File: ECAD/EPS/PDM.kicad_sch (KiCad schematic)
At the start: 12 parts, among them Q30 2N7002, Q31 IRF7458, U24 INA180A3

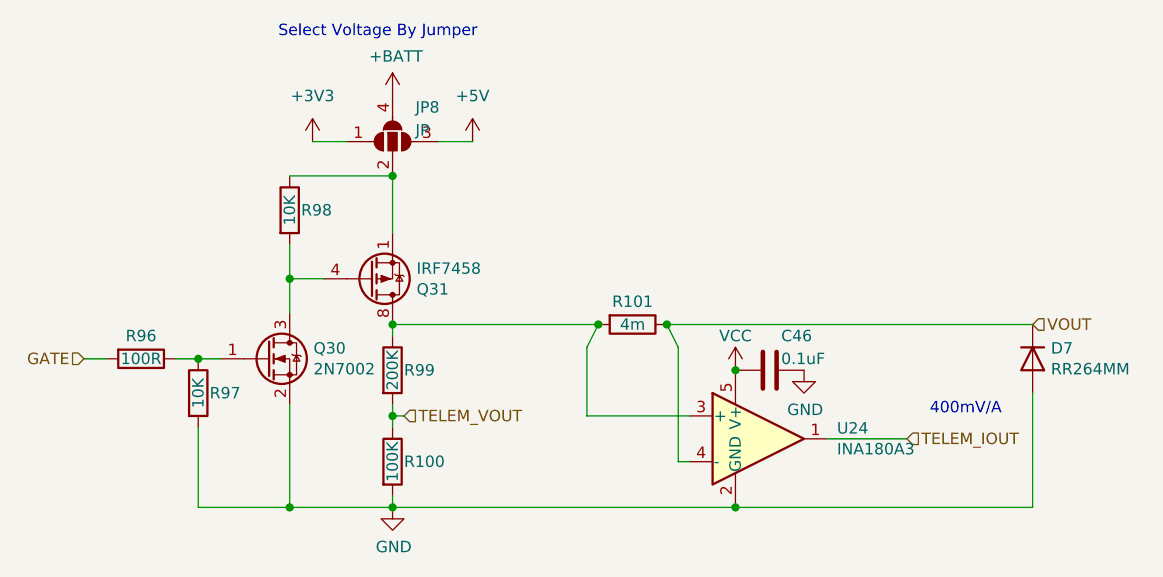
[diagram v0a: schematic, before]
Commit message: Micro + PCM blocks
Micro + PCM blocks
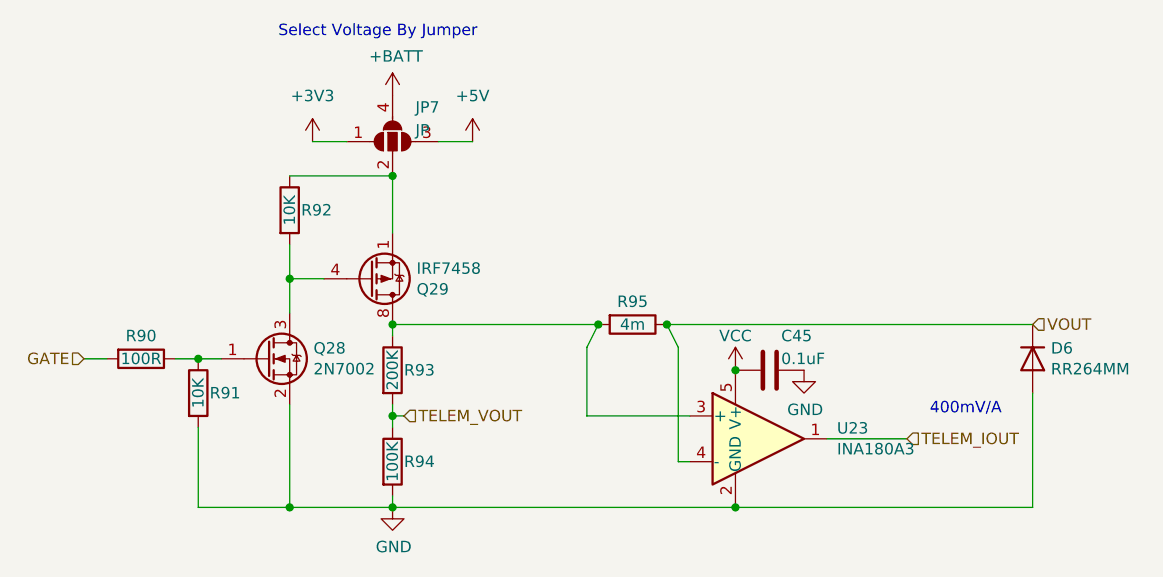
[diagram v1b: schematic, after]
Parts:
- renumbered C46 to C45, D7 to D6, JP8 to JP7, Q30 to Q28, Q31 to Q29, R96 to R90, R97 to R91, R98 to R92, R99 to R93, R100 to R94, R101 to R95, U24 to U23
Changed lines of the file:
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@@
     (effects (font (size 1.27 1.27)) (justify left))
   )
-  (symbol (lib_id "Device:D") (at 189.23 63.5 270) (unit 1)
-    (in_bom yes) (on_board yes)
-    (property "Reference" "D7" (id 0) (at 191.262 62.3316 90)
+  (symbol (lib_id "Device:D") (at 189.23 63.5 270)
+    (in_bom yes) (on_board yes)
+    (property "Reference" "D6" (id 0) (at 191.262 62.3316 90)
       (effects (font (size 1.27 1.27)) (justify left))
     )
@@
     (pin "2")
   )
-  (symbol (lib_id "Device:R") (at 118.11 64.77 0) (unit 1)
-    (in_bom yes) (on_board yes)
-    (property "Reference" "R99" (id 0) (at 119.38 64.77 0)
+  (symbol (lib_id "Device:R") (at 118.11 64.77 0)
+    (in_bom yes) (on_board yes)
+    (property "Reference" "R93" (id 0) (at 119.38 64.77 0)
       (effects (font (size 1.27 1.27)) (justify left))
     )
@@
     (pin "2")
   )
-  (symbol (lib_id "power:+BATT") (at 118.11 34.29 0) (unit 1)
-    (in_bom yes) (on_board yes)
-    (property "Reference" "#PWR0105" (id 0) (at 118.11 38.1 0)
+  (symbol (lib_id "power:+BATT") (at 118.11 34.29 0)
+    (in_bom yes) (on_board yes)
+    (property "Reference" "#PWR099" (id 0) (at 118.11 38.1 0)
       (effects (font (size 1.27 1.27)) hide)
     )
@@
     (pin "1")
   )
-  (symbol (lib_id "Transistor_FET:IRF7404") (at 115.57 54.61 0) (mirror x) (unit 1)
-    (in_bom yes) (on_board yes)
-    (property "Reference" "Q31" (id 0) (at 120.777 55.7784 0)
+  (symbol (lib_id "Transistor_FET:IRF7404") (at 115.57 54.61 0) (mirror x)
+    (in_bom yes) (on_board yes)
+    (property "Reference" "Q29" (id 0) (at 120.777 55.7784 0)
       (effects (font (size 1.27 1.27)) (justify left))
     )
@@
     (pin "8")
   )
-  (symbol (lib_id "Transistor_FET:2N7002") (at 104.14 63.5 0) (unit 1)
-    (in_bom yes) (on_board yes)
-    (property "Reference" "Q30" (id 0) (at 109.3216 62.3316 0)
+  (symbol (lib_id "Transistor_FET:2N7002") (at 104.14 63.5 0)
+    (in_bom yes) (on_board yes)
+    (property "Reference" "Q28" (id 0) (at 109.3216 62.3316 0)
       (effects (font (size 1.27 1.27)) (justify left))
     )
@@
     (pin "3")
   )
-  (symbol (lib_id "Device:R") (at 106.68 46.99 0) (unit 1)
-    (in_bom yes) (on_board yes)
-    (property "Reference" "R98" (id 0) (at 107.95 46.99 0)
+  (symbol (lib_id "Device:R") (at 106.68 46.99 0)
+    (in_bom yes) (on_board yes)
+    (property "Reference" "R92" (id 0) (at 107.95 46.99 0)
       (effects (font (size 1.27 1.27)) (justify left))
     )
@@
     (pin "2")
   )
-  (symbol (lib_id "Device:R") (at 90.17 63.5 270) (unit 1)
-    (in_bom yes) (on_board yes)
-    (property "Reference" "R96" (id 0) (at 90.17 60.96 90))
+  (symbol (lib_id "Device:R") (at 90.17 63.5 270)
+    (in_bom yes) (on_board yes)
+    (property "Reference" "R90" (id 0) (at 90.17 60.96 90))
     (property "Value" "100R" (id 1) (at 90.17 63.5 90))
     (property "Footprint" "" (id 2) (at 90.17 61.722 90)
@@
     (pin "2")
   )
-  (symbol (lib_id "Device:R") (at 96.52 67.31 0) (unit 1)
-    (in_bom yes) (on_board yes)
-    (property "Reference" "R97" (id 0) (at 97.79 67.31 0)
+  (symbol (lib_id "Device:R") (at 96.52 67.31 0)
+    (in_bom yes) (on_board yes)
+    (property "Reference" "R91" (id 0) (at 97.79 67.31 0)
       (effects (font (size 1.27 1.27)) (justify left))
     )
@@
     (pin "2")
   )
-  (symbol (lib_id "power:GND") (at 118.11 80.01 0) (unit 1)
-    (in_bom yes) (on_board yes)
-    (property "Reference" "#PWR0106" (id 0) (at 118.11 86.36 0)
+  (symbol (lib_id "power:GND") (at 118.11 80.01 0)
+    (in_bom yes) (on_board yes)
+    (property "Reference" "#PWR0100" (id 0) (at 118.11 86.36 0)
       (effects (font (size 1.27 1.27)) hide)
     )
@@
     (pin "1")
   )
-  (symbol (lib_id "Device:R") (at 144.78 59.69 270) (unit 1)
-    (in_bom yes) (on_board yes)
-    (property "Reference" "R101" (id 0) (at 144.78 57.15 90))
+  (symbol (lib_id "Device:R") (at 144.78 59.69 270)
+    (in_bom yes) (on_board yes)
+    (property "Reference" "R95" (id 0) (at 144.78 57.15 90))
     (property "Value" "4m" (id 1) (at 144.78 59.69 90))
     (property "Footprint" "Resistor_SMD:R_1206_3216Metric" (id 2) (at 144.78 57.912 90)
@@
     (pin "2")
   )
-  (symbol (lib_id "Device:R") (at 118.11 74.93 0) (unit 1)
-    (in_bom yes) (on_board yes)
-    (property "Reference" "R100" (id 0) (at 119.38 74.93 0)
+  (symbol (lib_id "Device:R") (at 118.11 74.93 0)
+    (in_bom yes) (on_board yes)
+    (property "Reference" "R94" (id 0) (at 119.38 74.93 0)
       (effects (font (size 1.27 1.27)) (justify left))
     )
@@
     (pin "2")
   )
-  (symbol (lib_id "Amplifier_Current:INA138") (at 158.75 72.39 0) (unit 1)
-    (in_bom yes) (on_board yes)
-    (property "Reference" "U24" (id 0) (at 167.4876 71.2216 0)
+  (symbol (lib_id "Amplifier_Current:INA138") (at 158.75 72.39 0)
+    (in_bom yes) (on_board yes)
+    (property "Reference" "U23" (id 0) (at 167.4876 71.2216 0)
       (effects (font (size 1.27 1.27)) (justify left))
     )
@@
     (pin "5")
   )
-  (symbol (lib_id "power:VCC") (at 156.21 64.77 0) (unit 1)
-    (in_bom yes) (on_board yes)
-    (property "Reference" "#PWR0108" (id 0) (at 156.21 68.58 0)
+  (symbol (lib_id "power:VCC") (at 156.21 64.77 0)
+    (in_bom yes) (on_board yes)
+    (property "Reference" "#PWR0102" (id 0) (at 156.21 68.58 0)
       (effects (font (size 1.27 1.27)) hide)
     )
@@
     (pin "1")
   )
-  (symbol (lib_id "Device:C") (at 160.02 64.77 90) (unit 1)
-    (in_bom yes) (on_board yes)
-    (property "Reference" "C46" (id 0) (at 161.29 60.96 90)
+  (symbol (lib_id "Device:C") (at 160.02 64.77 90)
+    (in_bom yes) (on_board yes)
+    (property "Reference" "C45" (id 0) (at 161.29 60.96 90)
       (effects (font (size 1.27 1.27)) (justify right))
     )
@@
     (pin "2")
   )
-  (symbol (lib_id "power:GND") (at 163.83 64.77 0) (unit 1)
-    (in_bom yes) (on_board yes)
-    (property "Reference" "#PWR0109" (id 0) (at 163.83 71.12 0)
+  (symbol (lib_id "power:GND") (at 163.83 64.77 0)
+    (in_bom yes) (on_board yes)
+    (property "Reference" "#PWR0103" (id 0) (at 163.83 71.12 0)
       (effects (font (size 1.27 1.27)) hide)
     )
@@
     (pin "1")
   )
-  (symbol (lib_id "symbols:SolderJumper_4_Open") (at 118.11 39.37 0) (unit 1)
-    (in_bom yes) (on_board yes)
-    (property "Reference" "JP8" (id 0) (at 120.65 35.56 0)
+  (symbol (lib_id "symbols:SolderJumper_4_Open") (at 118.11 39.37 0)
+    (in_bom yes) (on_board yes)
+    (property "Reference" "JP7" (id 0) (at 120.65 35.56 0)
       (effects (font (size 1.27 1.27)) (justify left))
     )
@@
     (pin "4")
   )
-  (symbol (lib_id "power:+5V") (at 127 39.37 0) (unit 1)
+  (symbol (lib_id "power:+5V") (at 127 39.37 0)
     (in_bom yes) (on_board yes) (fields_autoplaced)
-    (property "Reference" "#PWR0107" (id 0) (at 127 43.18 0)
+    (property "Reference" "#PWR0101" (id 0) (at 127 43.18 0)
       (effects (font (size 1.27 1.27)) hide)
     )
@@
     (pin "1")
   )
-  (symbol (lib_id "power:+3V3") (at 109.22 39.37 0) (unit 1)
+  (symbol (lib_id "power:+3V3") (at 109.22 39.37 0)
     (in_bom yes) (on_board yes) (fields_autoplaced)
-    (property "Reference" "#PWR0104" (id 0) (at 109.22 43.18 0)
-      (effects (font (size 1.27 1.27)) hide)
-    )
+    (property "Reference" "#PWR098" (id 0) (at 109.22 43.18 0)
+      (effects (font (size 1.27 1.27)) hide)
+    )

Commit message: Revert "Micro + PCM blocks"
This reverts commit bd53ca95fb26b4e6798500a23db46c8297649bcb.
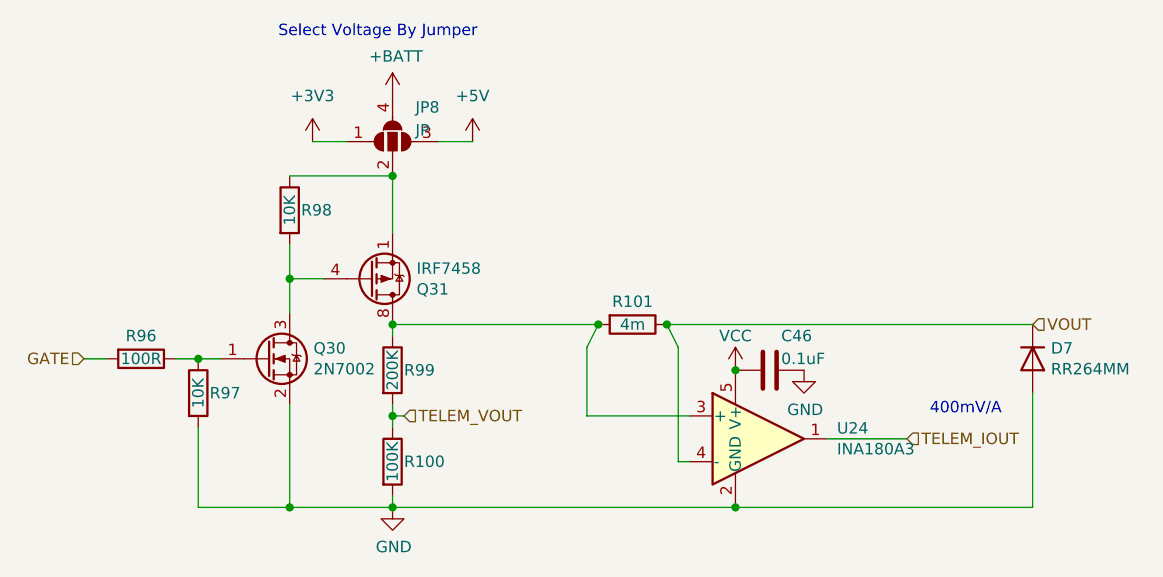
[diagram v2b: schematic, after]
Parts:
- renumbered C45 to C46, D6 to D7, JP7 to JP8, Q28 to Q30, Q29 to Q31, R94 to R100, R95 to R101, R90 to R96, R91 to R97, R92 to R98, R93 to R99, U23 to U24
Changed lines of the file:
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@@
     (effects (font (size 1.27 1.27)) (justify left))
   )
-  (symbol (lib_id "Device:D") (at 189.23 63.5 270)
-    (in_bom yes) (on_board yes)
-    (property "Reference" "D6" (id 0) (at 191.262 62.3316 90)
+  (symbol (lib_id "Device:D") (at 189.23 63.5 270) (unit 1)
+    (in_bom yes) (on_board yes)
+    (property "Reference" "D7" (id 0) (at 191.262 62.3316 90)
       (effects (font (size 1.27 1.27)) (justify left))
     )
@@
     (pin "2")
   )
-  (symbol (lib_id "Device:R") (at 118.11 64.77 0)
-    (in_bom yes) (on_board yes)
-    (property "Reference" "R93" (id 0) (at 119.38 64.77 0)
+  (symbol (lib_id "Device:R") (at 118.11 64.77 0) (unit 1)
+    (in_bom yes) (on_board yes)
+    (property "Reference" "R99" (id 0) (at 119.38 64.77 0)
       (effects (font (size 1.27 1.27)) (justify left))
     )
@@
     (pin "2")
   )
-  (symbol (lib_id "power:+BATT") (at 118.11 34.29 0)
-    (in_bom yes) (on_board yes)
-    (property "Reference" "#PWR099" (id 0) (at 118.11 38.1 0)
+  (symbol (lib_id "power:+BATT") (at 118.11 34.29 0) (unit 1)
+    (in_bom yes) (on_board yes)
+    (property "Reference" "#PWR0105" (id 0) (at 118.11 38.1 0)
       (effects (font (size 1.27 1.27)) hide)
     )
@@
     (pin "1")
   )
-  (symbol (lib_id "Transistor_FET:IRF7404") (at 115.57 54.61 0) (mirror x)
-    (in_bom yes) (on_board yes)
-    (property "Reference" "Q29" (id 0) (at 120.777 55.7784 0)
+  (symbol (lib_id "Transistor_FET:IRF7404") (at 115.57 54.61 0) (mirror x) (unit 1)
+    (in_bom yes) (on_board yes)
+    (property "Reference" "Q31" (id 0) (at 120.777 55.7784 0)
       (effects (font (size 1.27 1.27)) (justify left))
     )
@@
     (pin "8")
   )
-  (symbol (lib_id "Transistor_FET:2N7002") (at 104.14 63.5 0)
-    (in_bom yes) (on_board yes)
-    (property "Reference" "Q28" (id 0) (at 109.3216 62.3316 0)
+  (symbol (lib_id "Transistor_FET:2N7002") (at 104.14 63.5 0) (unit 1)
+    (in_bom yes) (on_board yes)
+    (property "Reference" "Q30" (id 0) (at 109.3216 62.3316 0)
       (effects (font (size 1.27 1.27)) (justify left))
     )
@@
     (pin "3")
   )
-  (symbol (lib_id "Device:R") (at 106.68 46.99 0)
-    (in_bom yes) (on_board yes)
-    (property "Reference" "R92" (id 0) (at 107.95 46.99 0)
+  (symbol (lib_id "Device:R") (at 106.68 46.99 0) (unit 1)
+    (in_bom yes) (on_board yes)
+    (property "Reference" "R98" (id 0) (at 107.95 46.99 0)
       (effects (font (size 1.27 1.27)) (justify left))
     )
@@
     (pin "2")
   )
-  (symbol (lib_id "Device:R") (at 90.17 63.5 270)
-    (in_bom yes) (on_board yes)
-    (property "Reference" "R90" (id 0) (at 90.17 60.96 90))
+  (symbol (lib_id "Device:R") (at 90.17 63.5 270) (unit 1)
+    (in_bom yes) (on_board yes)
+    (property "Reference" "R96" (id 0) (at 90.17 60.96 90))
     (property "Value" "100R" (id 1) (at 90.17 63.5 90))
     (property "Footprint" "" (id 2) (at 90.17 61.722 90)
@@
     (pin "2")
   )
-  (symbol (lib_id "Device:R") (at 96.52 67.31 0)
-    (in_bom yes) (on_board yes)
-    (property "Reference" "R91" (id 0) (at 97.79 67.31 0)
+  (symbol (lib_id "Device:R") (at 96.52 67.31 0) (unit 1)
+    (in_bom yes) (on_board yes)
+    (property "Reference" "R97" (id 0) (at 97.79 67.31 0)
       (effects (font (size 1.27 1.27)) (justify left))
     )
@@
     (pin "2")
   )
-  (symbol (lib_id "power:GND") (at 118.11 80.01 0)
-    (in_bom yes) (on_board yes)
-    (property "Reference" "#PWR0100" (id 0) (at 118.11 86.36 0)
+  (symbol (lib_id "power:GND") (at 118.11 80.01 0) (unit 1)
+    (in_bom yes) (on_board yes)
+    (property "Reference" "#PWR0106" (id 0) (at 118.11 86.36 0)
       (effects (font (size 1.27 1.27)) hide)
     )
@@
     (pin "1")
   )
-  (symbol (lib_id "Device:R") (at 144.78 59.69 270)
-    (in_bom yes) (on_board yes)
-    (property "Reference" "R95" (id 0) (at 144.78 57.15 90))
+  (symbol (lib_id "Device:R") (at 144.78 59.69 270) (unit 1)
+    (in_bom yes) (on_board yes)
+    (property "Reference" "R101" (id 0) (at 144.78 57.15 90))
     (property "Value" "4m" (id 1) (at 144.78 59.69 90))
     (property "Footprint" "Resistor_SMD:R_1206_3216Metric" (id 2) (at 144.78 57.912 90)
@@
     (pin "2")
   )
-  (symbol (lib_id "Device:R") (at 118.11 74.93 0)
-    (in_bom yes) (on_board yes)
-    (property "Reference" "R94" (id 0) (at 119.38 74.93 0)
+  (symbol (lib_id "Device:R") (at 118.11 74.93 0) (unit 1)
+    (in_bom yes) (on_board yes)
+    (property "Reference" "R100" (id 0) (at 119.38 74.93 0)
       (effects (font (size 1.27 1.27)) (justify left))
     )
@@
     (pin "2")
   )
-  (symbol (lib_id "Amplifier_Current:INA138") (at 158.75 72.39 0)
-    (in_bom yes) (on_board yes)
-    (property "Reference" "U23" (id 0) (at 167.4876 71.2216 0)
+  (symbol (lib_id "Amplifier_Current:INA138") (at 158.75 72.39 0) (unit 1)
+    (in_bom yes) (on_board yes)
+    (property "Reference" "U24" (id 0) (at 167.4876 71.2216 0)
       (effects (font (size 1.27 1.27)) (justify left))
     )
@@
     (pin "5")
   )
-  (symbol (lib_id "power:VCC") (at 156.21 64.77 0)
-    (in_bom yes) (on_board yes)
-    (property "Reference" "#PWR0102" (id 0) (at 156.21 68.58 0)
+  (symbol (lib_id "power:VCC") (at 156.21 64.77 0) (unit 1)
+    (in_bom yes) (on_board yes)
+    (property "Reference" "#PWR0108" (id 0) (at 156.21 68.58 0)
       (effects (font (size 1.27 1.27)) hide)
     )
@@
     (pin "1")
   )
-  (symbol (lib_id "Device:C") (at 160.02 64.77 90)
-    (in_bom yes) (on_board yes)
-    (property "Reference" "C45" (id 0) (at 161.29 60.96 90)
+  (symbol (lib_id "Device:C") (at 160.02 64.77 90) (unit 1)
+    (in_bom yes) (on_board yes)
+    (property "Reference" "C46" (id 0) (at 161.29 60.96 90)
       (effects (font (size 1.27 1.27)) (justify right))
     )
@@
     (pin "2")
   )
-  (symbol (lib_id "power:GND") (at 163.83 64.77 0)
-    (in_bom yes) (on_board yes)
-    (property "Reference" "#PWR0103" (id 0) (at 163.83 71.12 0)
+  (symbol (lib_id "power:GND") (at 163.83 64.77 0) (unit 1)
+    (in_bom yes) (on_board yes)
+    (property "Reference" "#PWR0109" (id 0) (at 163.83 71.12 0)
       (effects (font (size 1.27 1.27)) hide)
     )
@@
     (pin "1")
   )
-  (symbol (lib_id "symbols:SolderJumper_4_Open") (at 118.11 39.37 0)
-    (in_bom yes) (on_board yes)
-    (property "Reference" "JP7" (id 0) (at 120.65 35.56 0)
+  (symbol (lib_id "symbols:SolderJumper_4_Open") (at 118.11 39.37 0) (unit 1)
+    (in_bom yes) (on_board yes)
+    (property "Reference" "JP8" (id 0) (at 120.65 35.56 0)
       (effects (font (size 1.27 1.27)) (justify left))
     )
@@
     (pin "4")
   )
-  (symbol (lib_id "power:+5V") (at 127 39.37 0)
+  (symbol (lib_id "power:+5V") (at 127 39.37 0) (unit 1)
     (in_bom yes) (on_board yes) (fields_autoplaced)
-    (property "Reference" "#PWR0101" (id 0) (at 127 43.18 0)
+    (property "Reference" "#PWR0107" (id 0) (at 127 43.18 0)
       (effects (font (size 1.27 1.27)) hide)
     )
@@
     (pin "1")
   )
-  (symbol (lib_id "power:+3V3") (at 109.22 39.37 0)
+  (symbol (lib_id "power:+3V3") (at 109.22 39.37 0) (unit 1)
     (in_bom yes) (on_board yes) (fields_autoplaced)
-    (property "Reference" "#PWR098" (id 0) (at 109.22 43.18 0)
-      (effects (font (size 1.27 1.27)) hide)
-    )
+    (property "Reference" "#PWR0104" (id 0) (at 109.22 43.18 0)
+      (effects (font (size 1.27 1.27)) hide)
+    )
